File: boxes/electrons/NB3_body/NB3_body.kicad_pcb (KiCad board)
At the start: 2 copper layers, 200 x 199.5 mm, 39 parts, among them J1 Conn_02x05_Counter_Clockwise, J10 Conn_02x03_Top_Bottom, J11 Conn_02x03_Top_Bottom, J12 Conn_02x03_Top_Bottom, J13 JST ZH 6-way Socket, J14 JST ZH 6-way Socket, J15 Conn_02x03_Top_Bottom, J16 Conn_02x03_Top_Bottom, J2 Conn_02x05_Counter_Clockwise, J3 Conn_02x05_Counter_Clockwise, J4 Conn_02x05_Counter_Clockwise, J5 Conn_02x05_Counter_Clockwise, J6 Conn_02x05_Counter_Clockwise, J7 Conn_02x05_Counter_Clockwise, J8 Conn_02x05_Counter_Clockwise, J9 JST SH 4-way Socket

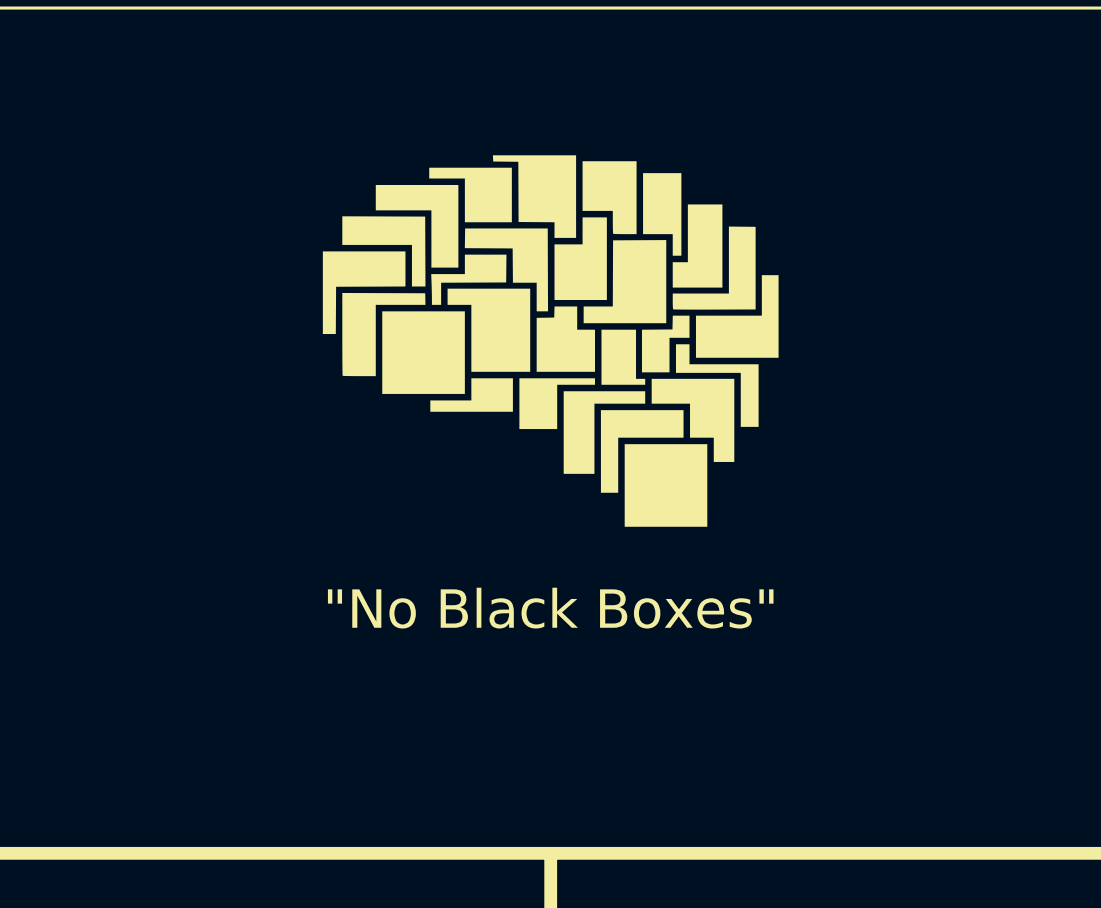
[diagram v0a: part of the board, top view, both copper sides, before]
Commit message: Update NB3 PCBs and parts
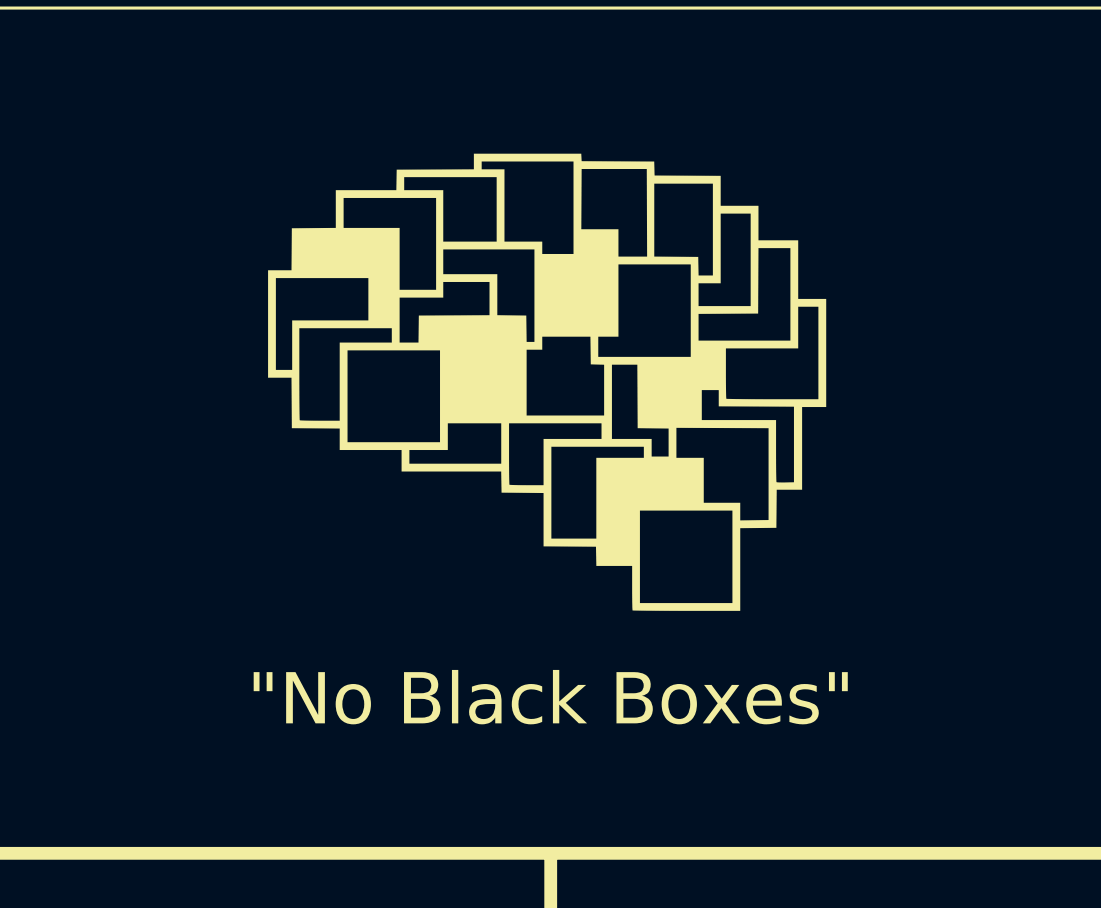
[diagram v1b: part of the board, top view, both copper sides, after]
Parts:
- removed the G*** at (124.5, 116.0)
- added G***: LOGO, NB3_body:Logo_NBB_30mm, F.Cu at (124.5, 117.0)
